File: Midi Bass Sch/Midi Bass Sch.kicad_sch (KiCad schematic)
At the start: 4 parts

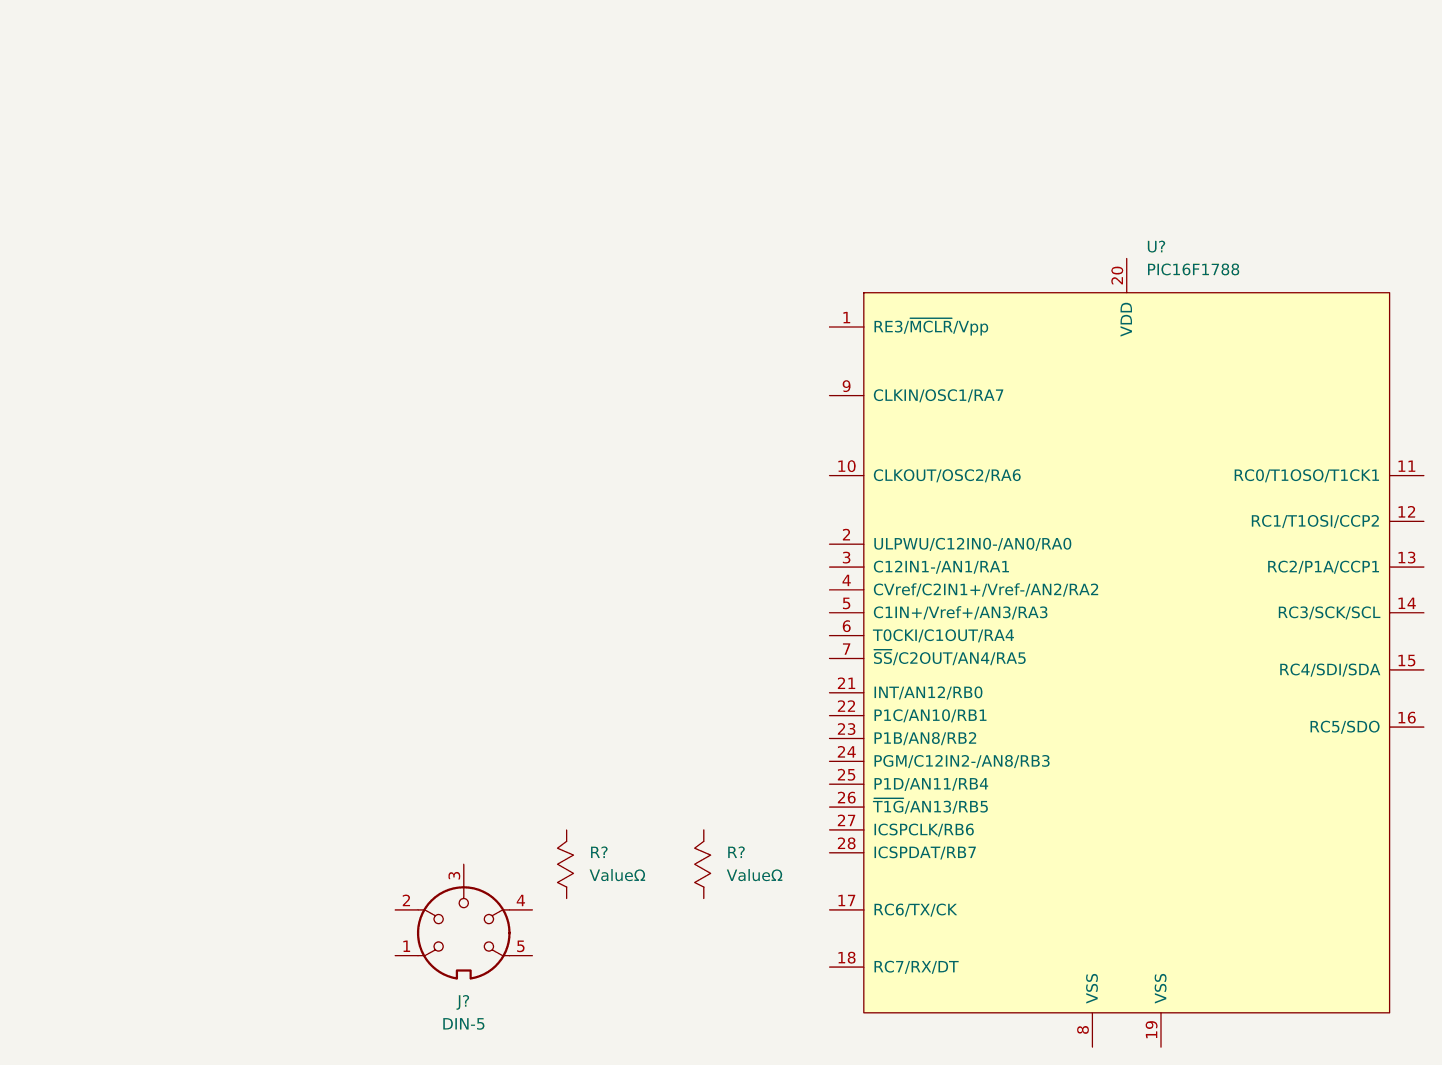
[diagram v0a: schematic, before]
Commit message: updated schematic
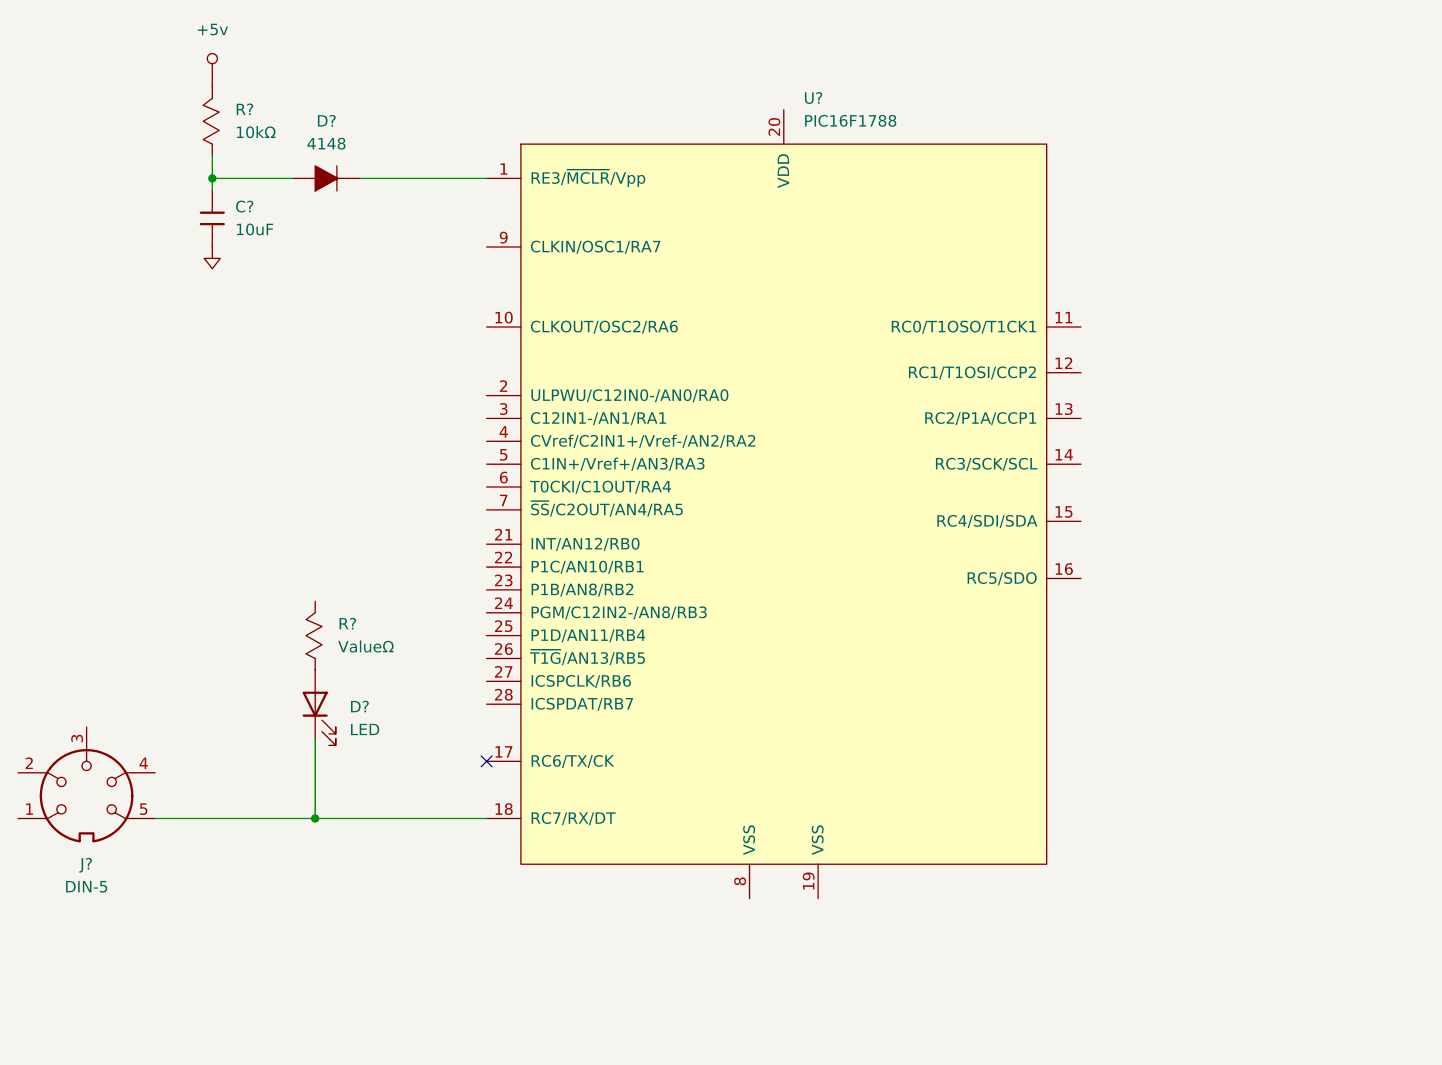
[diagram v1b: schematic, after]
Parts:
- removed R?: ValueΩ, symbol Owen's Symbols:Resistor_Mod
- added C?: 10uF, symbol Owen's Symbols:Capacitor
- added D?: LED, symbol Device:LED
- added D?: 4148, symbol Owen's Symbols:Diode
- added R?: 10kΩ, symbol Owen's Symbols:Resistor_Mod
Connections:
- net at U?.1 (RE3/~{MCLR}/Vpp): now also D?.2
- net at J?.5: now also D?.1 (K)
- net at R?.1: now also D?.2 (A)
- new net: C?.1, D?.1, R?.1
- new net +5v: R?.2
- new net GND: C?.2
- no-connect marks 0 -> 1
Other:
- moved on the sheet: J?, R?, U?
